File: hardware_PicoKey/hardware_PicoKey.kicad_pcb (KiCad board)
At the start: 2 copper layers, 34.5 x 18.5 mm, 36 parts, among them J1 USB_A, SW1 SW_Push, SW2 SW_Push, U1 RP2350A-QFN60, U2 AMS1117S-3.3, U3 W25Q128JVS, Y1 Crystal_GND24

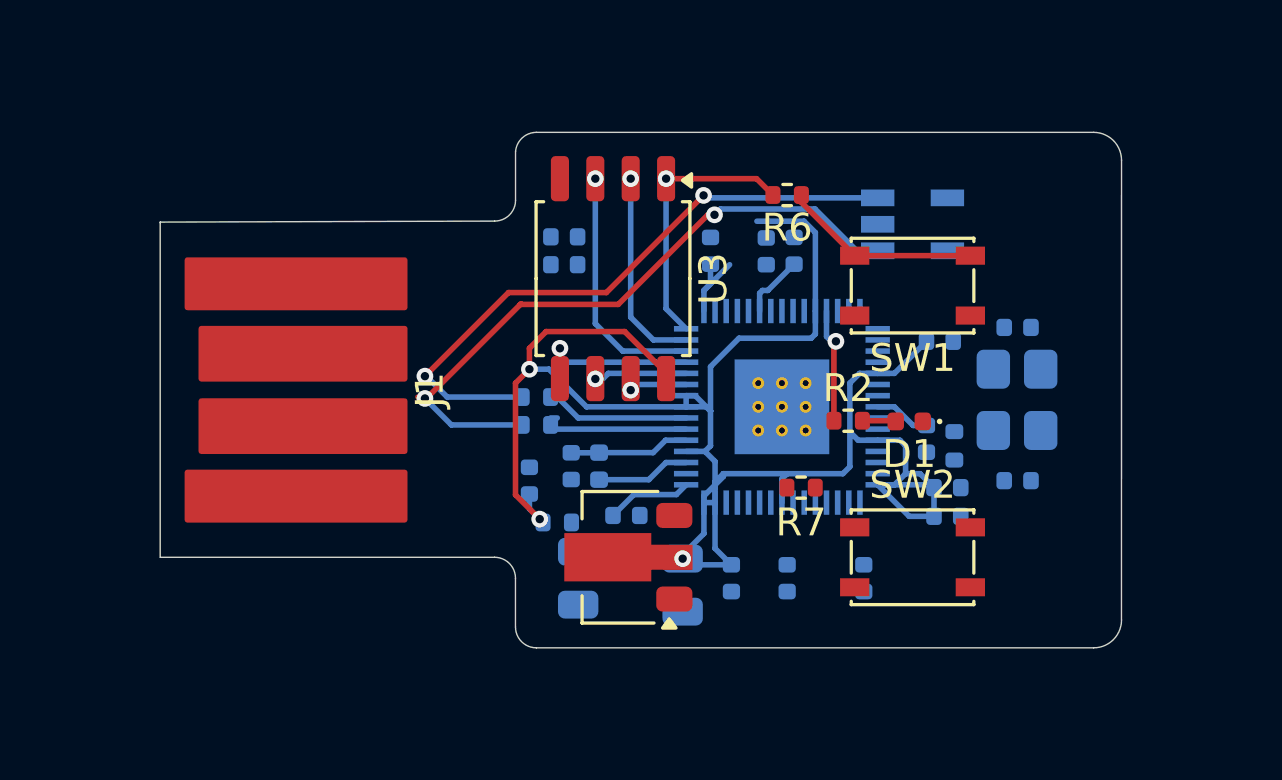
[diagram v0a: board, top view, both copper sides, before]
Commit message: pcb
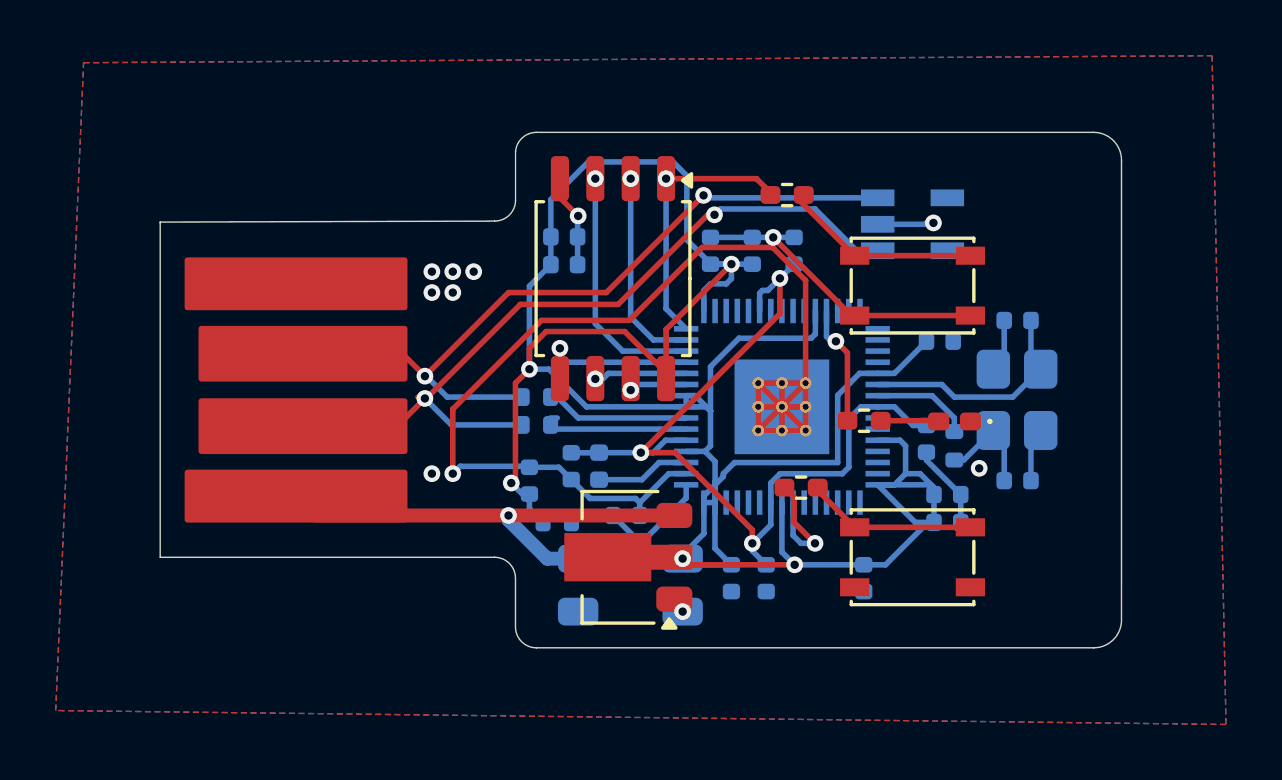
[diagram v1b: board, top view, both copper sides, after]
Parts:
- D1: footprint LED_SMD:LED_0402_1005Metric -> LED_SMD:LED_0402_1005Metric_Pad0.77x0.64mm_HandSolder
- R2, R6, R7: footprint Resistor_SMD:R_0402_1005Metric -> Resistor_SMD:R_0402_1005Metric_Pad0.72x0.64mm_HandSolder
- moved D1 1.63 mm to (151.5, 69.6)
- moved C8 0.75 mm to (144.8, 75.2)
- moved R2 0.57 mm to (148.3, 69.6)
- moved C11 0.50 mm to (144.2, 63.5)
- moved C14 0.25 mm to (151.2, 72.2)
- moved C19 0.25 mm to (153.8, 66.0)
- moved C4 0.25 mm to (138.0, 75.5)
- moved C13 0.22 mm to (151.2, 73.2)
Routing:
- net GND: track 0.00 -> 70.0 mm, vias 0 -> 12
- net 3v3: track 73.9 -> 99.4 mm, vias 3 -> 5
- net 1v1: track 8.65 -> 32.0 mm, vias 0 -> 3
- net Net-(J1-VBUS): track 0.00 -> 17.1 mm, vias 0 -> 1
- net XIN: track 0.00 -> 8.10 mm
- net Net-(R7-Pad2): track 0.00 -> 6.12 mm
- net USB_DM: track 23.9 -> 28.7 mm
- net USB_DP: track 23.9 -> 28.7 mm
- net Net-(U1-GPIO25): track 0.00 -> 4.54 mm, vias 0 -> 1
- net Net-(C18-Pad1): track 0.00 -> 3.80 mm
- net XOUT: track 0.00 -> 3.57 mm
- net Net-(U1-VREG_AVDD): track 3.08 -> 5.57 mm
- net Net-(D1-A): track 1.21 -> 2.09 mm
- added copper zone on B.Cu, net GND
- added copper zone on F.Cu, net GND
